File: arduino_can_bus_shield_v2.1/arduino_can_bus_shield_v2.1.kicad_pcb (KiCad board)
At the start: 2 copper layers, 68.6 x 53.3 mm, 36 parts, among them J1 Power, J2 Digital/PWM, J3 Analog, J4 Digital/PWM, J6 xt60 male, J7 molex_3.0, M1 MPU9250_module, SW1 User, SW2 User, SW3 SW_DIP_x04, U1 MP1584, U2 MCP2551-I-SN, U3 MCP2515-xST, Y1 16MHz

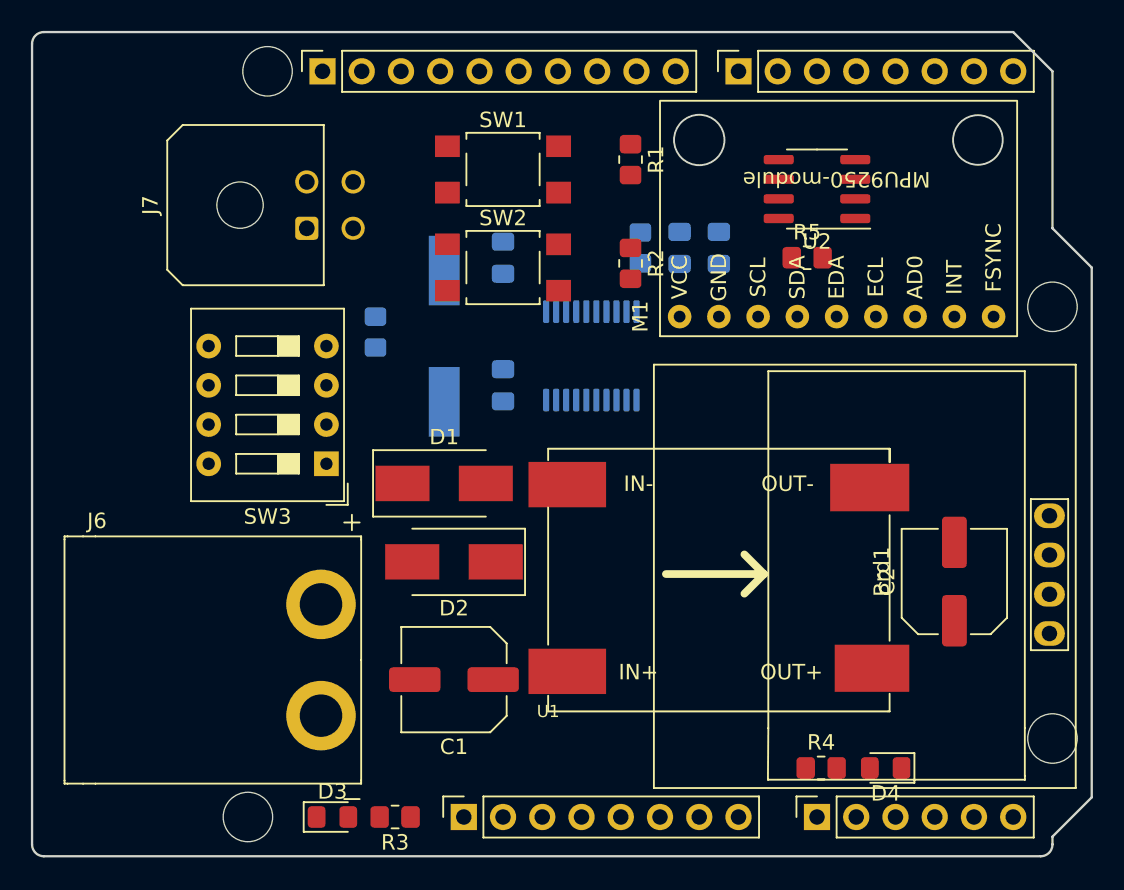
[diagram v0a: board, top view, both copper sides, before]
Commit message: Add files via upload
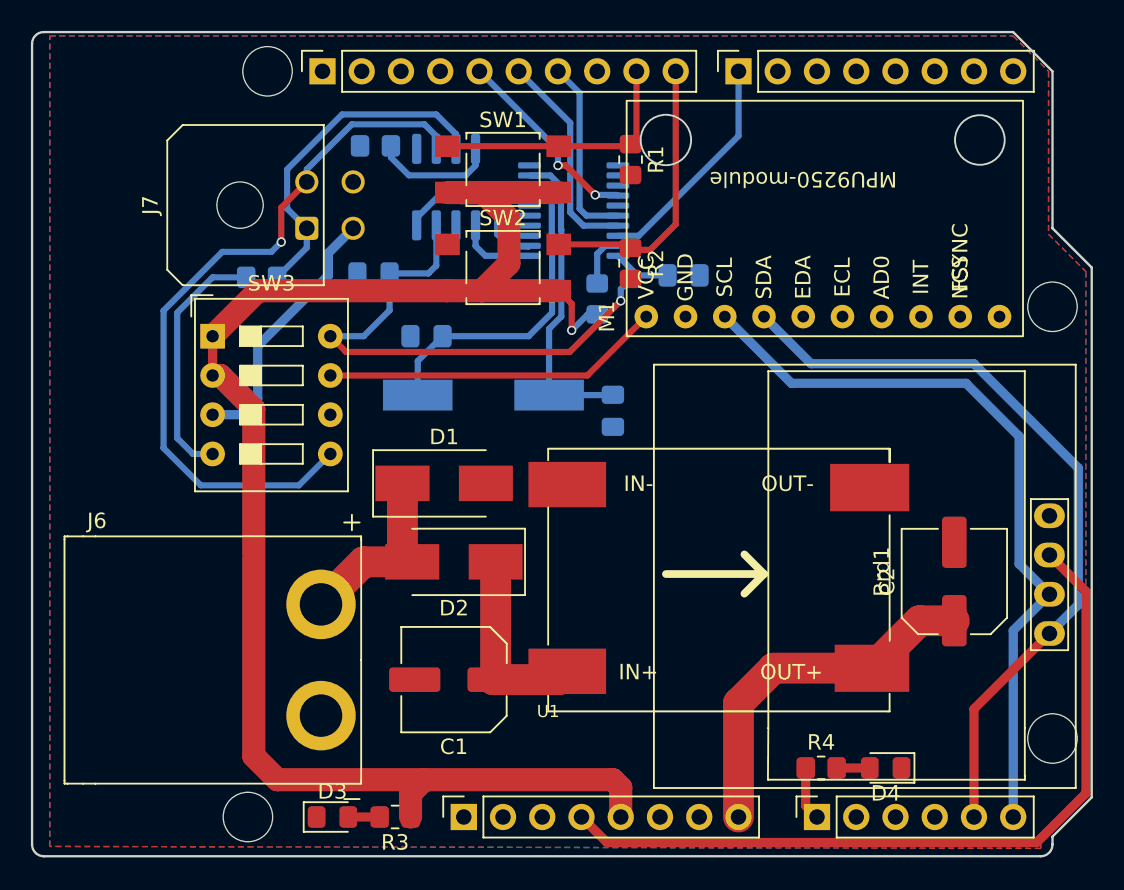
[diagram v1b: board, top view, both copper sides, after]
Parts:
- R5, U2: moved to B.Cu
- moved R5 28.9 mm to (122.2, 54.0), turned to 180 degrees
- moved U2 24.0 mm to (126.8, 56.7), turned to 90 degrees
- moved C6 19.9 mm to (122.1, 62.3), turned to 180 degrees
- moved SW3 11.1 mm to (111.7, 66.3), turned to 0 degrees
- moved U3 9.47 mm to (135.1, 58.2), turned to 0 degrees
- moved R6 8.17 mm to (114.9, 62.5), turned to 180 degrees
- moved C5 7.30 mm to (137.6, 71.2), turned to -90 degrees
- moved C3 7.09 mm to (125.5, 66.3), turned to 180 degrees
- moved Y1 4.58 mm to (129.2, 70.2), turned to 0 degrees
- moved R7 4.33 mm to (136.6, 63.9)
- moved C4 2.90 mm to (142.2, 62.4), turned to 0 degrees
- moved M1 2.16 mm to (149.9, 58.7)
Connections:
- Brd1 pad 2: +3.3V -> +3V3
- Brd1 pad 3: /A5(SCL) -> /SCL/A5
- Brd1 pad 4: /A4(SDA) -> /SDA/A4
- J2 pad 5: /13 -> /13(SCK)
- J2 pad 6: /12 -> /12(MISO)
- J2 pad 7: /*11 -> /11(**/MOSI)
- J2 pad 9: /*9 -> /9(**)
- M1 pad 2: /A5(SCL) -> /SCL/A5
- M1 pad 3: /A4(SDA) -> /SDA/A4
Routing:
- net +5V: track 0.00 -> 102.8 mm, vias 0 -> 1
- net +3V3: track 0.00 -> 51.0 mm
- net /SDA/A4: track 0.00 -> 49.8 mm
- net /SCL/A5: track 0.00 -> 48.7 mm
- net /CAN-: track 0.00 -> 47.1 mm, vias 0 -> 1
- net /can_enable: track 0.00 -> 39.3 mm, vias 0 -> 1
- net VCC: track 0.00 -> 23.5 mm
- net /CAN+: track 0.00 -> 22.2 mm
- net /imu_enable: track 0.00 -> 22.0 mm
- net Net-(C3-Pad1): track 0.00 -> 21.5 mm
- net Net-(C5-Pad1): track 0.00 -> 20.3 mm
- net /8: track 0.00 -> 18.3 mm
- net Net-(J7-Pad3): track 0.00 -> 16.9 mm
- net /9(**): track 0.00 -> 16.8 mm
- net Net-(R6-Pad2): track 0.00 -> 16.2 mm
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- added copper zone on B.Cu, net GND
- added copper zone on F.Cu, net GND
